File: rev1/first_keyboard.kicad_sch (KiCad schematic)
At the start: 83 parts, among them SW1 SW_Push, SW10 SW_Push, SW11 SW_Push, SW12 SW_Push, SW13 SW_Push, SW14 SW_Push, SW15 SW_Push, SW16 SW_Push, SW17 SW_Push, SW18 SW_Push, SW19 SW_Push, SW2 SW_Push, SW20 SW_Push, SW21 SW_Push, SW22 SW_Push, SW23 SW_Push, SW24 SW_Push, SW25 SW_Push, SW26 SW_Push, SW27 SW_Push, SW28 SW_Push, SW29 SW_Push, SW3 SW_Push, SW30 SW_Push, SW31 SW_Push, SW32 SW_Push, SW33 SW_Push, SW34 SW_Push, SW35 SW_Push, SW36 SW_Push, SW37 SW_Push, SW38 SW_Push, SW39 SW_Push, SW4 SW_Push, SW40 SW_Push, SW41 SW_Push, SW5 SW_Push, SW6 SW_Push, SW7 SW_Push, SW8 SW_Push, SW9 SW_Push, U1 Pico

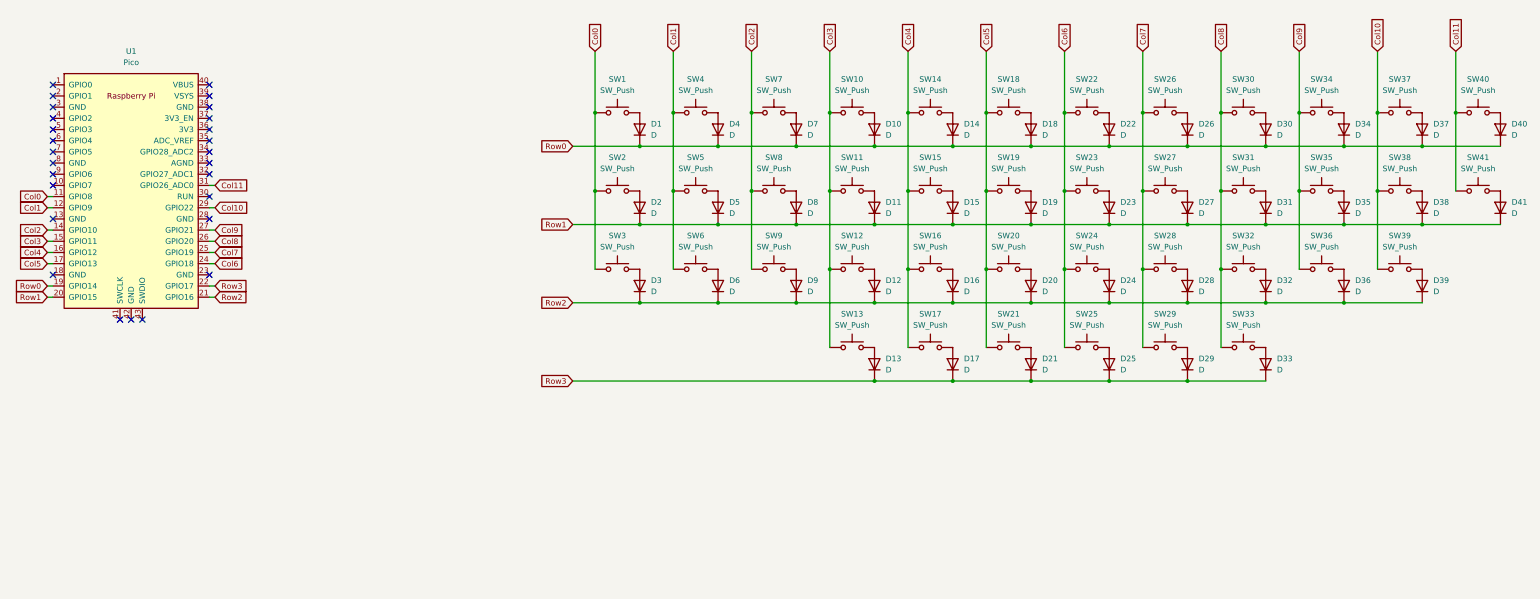
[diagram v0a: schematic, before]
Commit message: feat: スイッチとダイオードは置いた
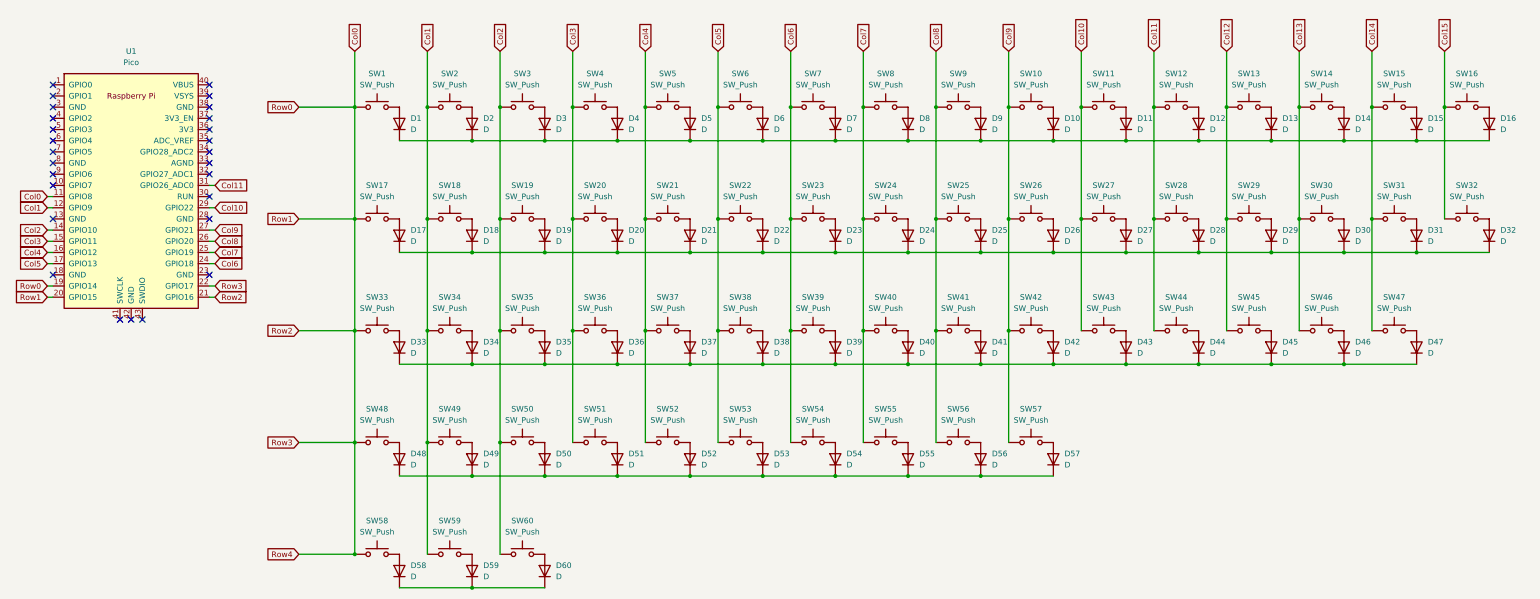
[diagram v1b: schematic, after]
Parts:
- added D42, D43, D44, D45, D46, D47, D48, D49, D50, D51, D52, D53, D54, D55, D56, D57, D58, D59, D60: D, symbol Device:D
- added SW42, SW43, SW44, SW45, SW46, SW47, SW48, SW49, SW50, SW51, SW52, SW53, SW54, SW55, SW56, SW57, SW58, SW59, SW60: SW_Push, symbol Switch:SW_Push
- D1, D10, D11, D12, D13, D14, D15, D16, D17, D18, D19, D2, D20, D21, D22, D23, D24, D25, D26, D27, D28, D29, D3, D30, D31, D32, D33, D34, D35, D36, D37, D38, D39, D4, D40, D41, D5, D6, D7, D8, D9: footprint kbd_Parts:Diode_TH_SMD -> (none)
- SW1, SW10, SW11, SW12, SW13, SW14, SW15, SW16, SW17, SW18, SW19, SW2, SW20, SW21, SW22, SW23, SW24, SW25, SW26, SW27, SW28, SW29, SW3, SW30, SW31, SW32, SW33, SW34, SW35, SW36, SW37, SW38, SW39, SW4, SW40, SW5, SW6, SW7, SW8, SW9: footprint kbd_SW:CherryMX_Hotswap_1u -> (none)
- SW41: footprint kbd_SW:CherryMX_Hotswap_2u -> (none)
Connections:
- net Col0: now also SW17.1, SW33.1, U1.19 (GPIO14), U1.20 (GPIO15), U1.21 (GPIO16), U1.22 (GPIO17), SW48.1, SW58.1; no longer SW2.1, SW3.1
- net Col1: now also SW18.1, SW2.1, SW34.1, SW49.1, SW59.1; no longer SW4.1, SW5.1, SW6.1
- net Col10: now also SW11.1, SW27.1, SW43.1; no longer SW37.1, SW38.1, SW39.1
- net Col11: now also SW12.1, SW28.1, SW44.1; no longer SW40.1, SW41.1
- net Col2: now also SW19.1, SW3.1, SW35.1, SW50.1, SW60.1; no longer SW7.1, SW8.1, SW9.1
- net Col3: now also SW20.1, SW36.1, SW4.1, SW51.1; no longer SW10.1, SW11.1, SW12.1, SW13.1
- net Col4: now also SW21.1, SW37.1, SW5.1, SW52.1; no longer SW14.1, SW15.1, SW16.1, SW17.1
- net Col5: now also SW22.1, SW38.1, SW6.1, SW53.1; no longer SW18.1, SW19.1, SW20.1, SW21.1
- net Col6: now also SW39.1, SW7.1, SW54.1; no longer SW22.1, SW24.1, SW25.1
- net Col7: now also SW24.1, SW40.1, SW8.1, SW55.1; no longer SW26.1, SW27.1, SW28.1, SW29.1
- net Col8: now also SW25.1, SW41.1, SW9.1, SW56.1; no longer SW30.1, SW31.1, SW32.1, SW33.1
- net Col9: now also SW10.1, SW26.1, SW42.1, SW57.1; no longer SW34.1, SW35.1, SW36.1
- removed net Row0: D1.1 (K), D10.1 (K), D14.1 (K), D18.1 (K), D22.1 (K), D26.1 (K), D30.1 (K), D34.1 (K), D37.1 (K), D4.1 (K), D40.1 (K), D7.1 (K), U1.19 (GPIO14)
- removed net Row1: D11.1 (K), D15.1 (K), D19.1 (K), D2.1 (K), D23.1 (K), D27.1 (K), D31.1 (K), D35.1 (K), D38.1 (K), D41.1 (K), D5.1 (K), D8.1 (K), U1.20 (GPIO15)
- removed net Row2: D12.1 (K), D16.1 (K), D20.1 (K), D24.1 (K), D28.1 (K), D3.1 (K), D32.1 (K), D36.1 (K), D39.1 (K), D6.1 (K), D9.1 (K), U1.21 (GPIO16)
- net Row3: no longer names the net of D17.1 (K), D21.1 (K), D25.1 (K), D29.1 (K)
- net Row3: now also D18.1 (K), D19.1 (K), D20.1 (K), D22.1 (K), D23.1 (K), D24.1 (K), D26.1 (K), D27.1 (K), D28.1 (K), D30.1 (K), D31.1 (K), D32.1 (K); no longer D13.1 (K), D33.1 (K), U1.22 (GPIO17)
- new net: D33.1 (K), D34.1 (K), D35.1 (K), D36.1 (K), D37.1 (K), D38.1 (K), D39.1 (K), D40.1 (K), D41.1 (K), D42.1 (K), D43.1 (K), D44.1 (K), D45.1 (K), D46.1 (K), D47.1 (K)
- new net: D42.2 (A), SW42.2
- new net: D58.1 (K), D59.1 (K), D60.1 (K)
- new net: D60.2 (A), SW60.2
- new net: D51.2 (A), SW51.2
- new net: D44.2 (A), SW44.2
- new net: D1.1 (K), D10.1 (K), D11.1 (K), D12.1 (K), D13.1 (K), D14.1 (K), D15.1 (K), D16.1 (K), D2.1 (K), D3.1 (K), D4.1 (K), D5.1 (K), D6.1 (K), D7.1 (K), D8.1 (K), D9.1 (K)
- new net: D46.2 (A), SW46.2
- new net: D43.2 (A), SW43.2
- new net: D49.2 (A), SW49.2
- new net: D58.2 (A), SW58.2
- new net: D59.2 (A), SW59.2
- new net: D55.2 (A), SW55.2
- new net: D48.1 (K), D49.1 (K), D50.1 (K), D51.1 (K), D52.1 (K), D53.1 (K), D54.1 (K), D55.1 (K), D56.1 (K), D57.1 (K)
- new net: D53.2 (A), SW53.2
- new net: D45.2 (A), SW45.2
- new net: D48.2 (A), SW48.2
- new net: D50.2 (A), SW50.2
- new net: D57.2 (A), SW57.2
- new net: D47.2 (A), SW47.2
- new net: D52.2 (A), SW52.2
- new net: D54.2 (A), SW54.2
- new net: D56.2 (A), SW56.2
- new net Col12: SW13.1, SW29.1, SW45.1
- new net Col13: SW14.1, SW30.1, SW46.1
- new net Col14: SW15.1, SW31.1, SW47.1
- new net Col15: SW16.1, SW32.1
